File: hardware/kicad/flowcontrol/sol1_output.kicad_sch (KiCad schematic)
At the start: 9 parts, among them J3 SOL1_PORT, Q1 SOL1_NFET

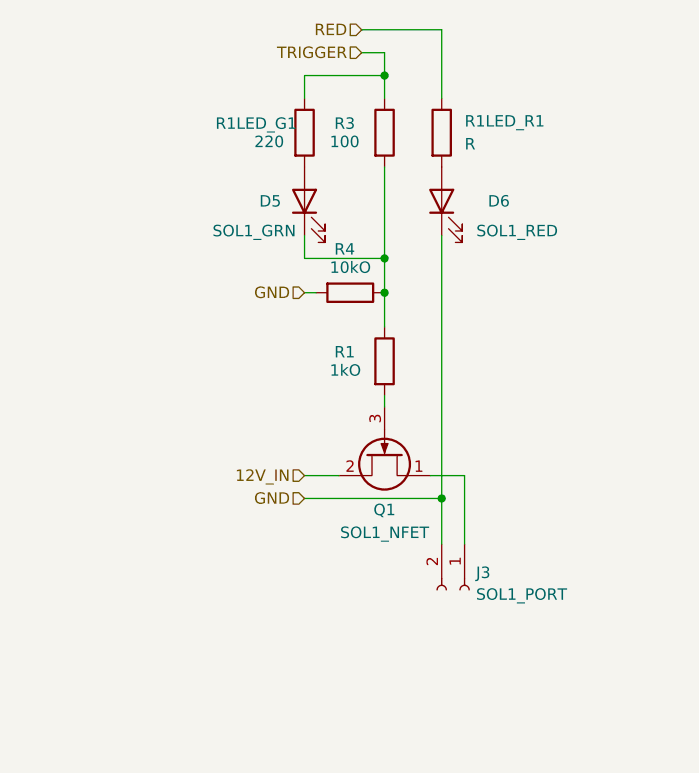
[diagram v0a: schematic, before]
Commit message: Updated KiCad schematic to final rendition
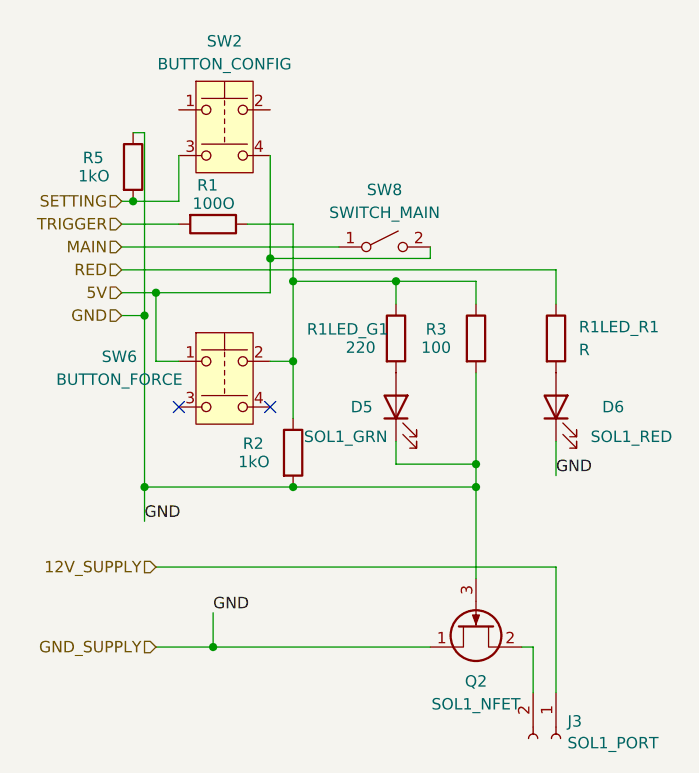
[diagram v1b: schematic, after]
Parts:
- removed R4: 10kO, Resistor_THT:R_Axial_DIN0309_L9.0mm_D3.2mm_P15.24mm_Horizontal, symbol Device:R
- added R2, R5: 1kO, Resistor_THT:R_Axial_DIN0309_L9.0mm_D3.2mm_P15.24mm_Horizontal, symbol Device:R
- added SW2: BUTTON_CONFIG, symbol Switch:SW_Push_Dual
- added SW6: BUTTON_FORCE, symbol Switch:SW_Push_Dual
- added SW8: SWITCH_MAIN, symbol Switch:SW_SPST
- R1: value 1kO -> 100O
- renumbered Q1 to Q2
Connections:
- net GND: now also D5.1 (K), Q2.1 (D), Q2.3 (G), R3.2, R2.2, R5.1; no longer J3.2 (Pin_2)
- net TRIGGER: now also R1.2; no longer R1LED_G1.1, R3.1
- net 12V_SUPPLY: now reaches J3.1 (Pin_1)
- net 12V_SUPPLY: no longer Q2.1 (D)
- net 12V_IN: no longer names the net of Q2.2 (S)
- net 12V_IN: now also J3.2 (Pin_2)
- new net: R1.1, R1LED_G1.1, R2.1, R3.1, SW6.2
- new net 5V: SW2.4, SW6.1, SW8.2 (B)
- new net MAIN: SW8.1 (A)
- new net SETTING: R5.2, SW2.3
- no-connect marks 0 -> 2
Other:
- moved on the sheet: D5, D6, J3, Q2, R1, R1LED_G1, R1LED_R1, R3
